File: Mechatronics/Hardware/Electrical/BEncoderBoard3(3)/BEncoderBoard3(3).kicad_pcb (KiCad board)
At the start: 4 copper layers, 34 x 33 mm, 10 parts, among them J1 Conn_01x04_Male, U8 RN4871U

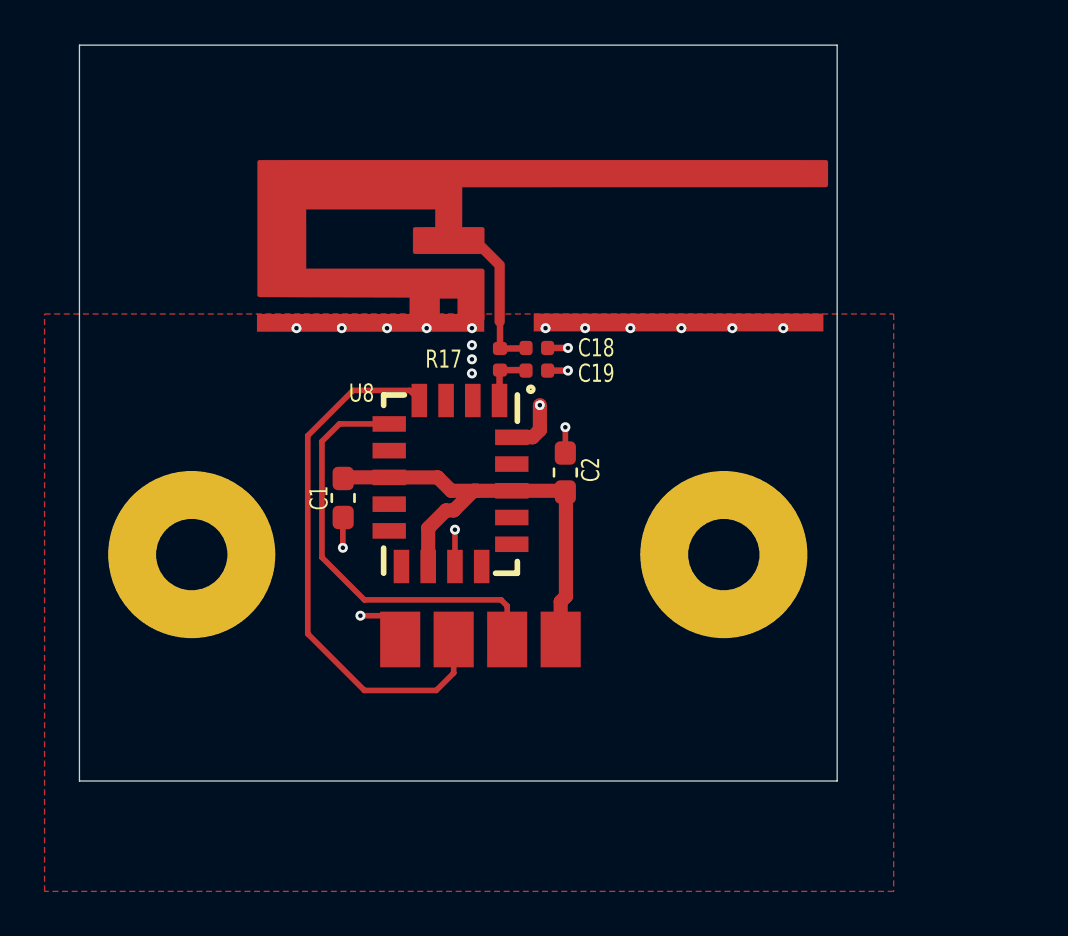
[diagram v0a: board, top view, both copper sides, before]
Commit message: PCB changes
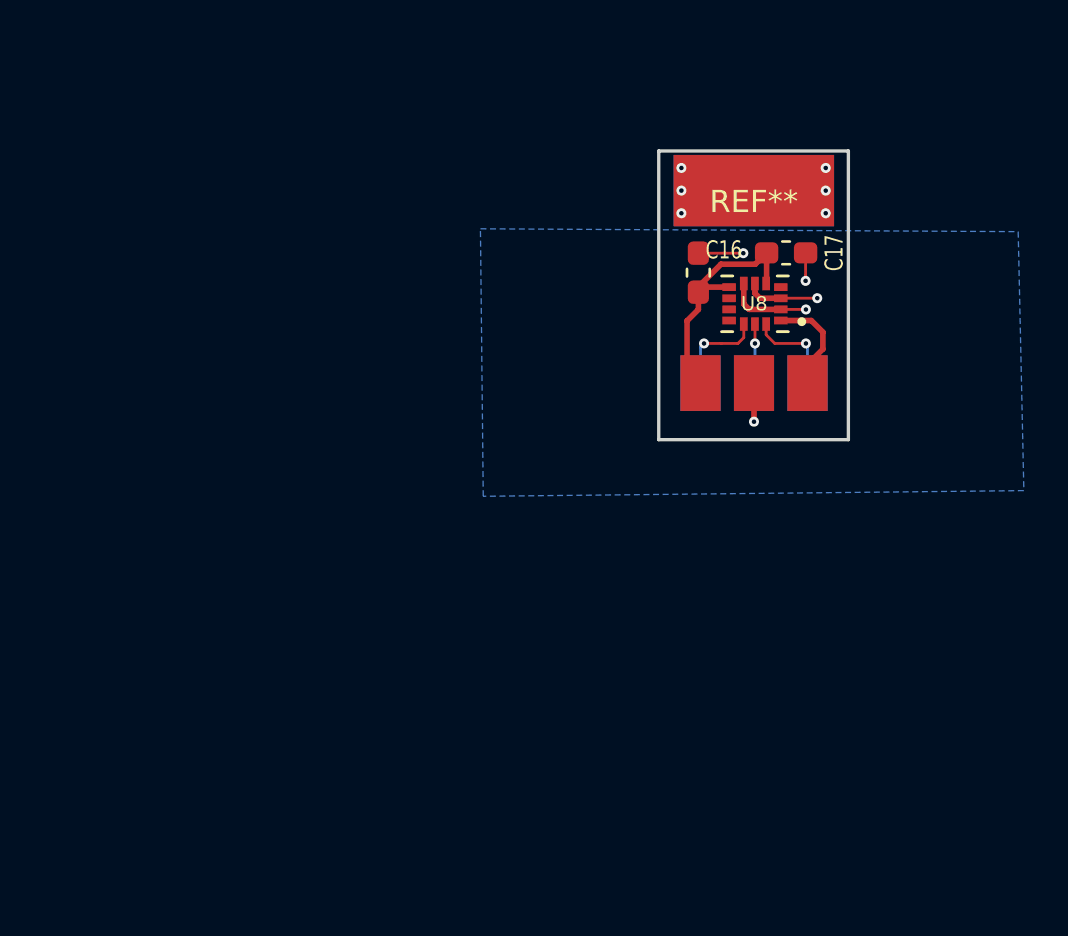
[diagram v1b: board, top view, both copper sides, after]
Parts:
- removed AE1: LOGO, Encoder:Antenna
- removed C1: 1uF, Encoder:C_0603_1608Metric_Pad1.05x0.95mm_HandSolder
- removed C18, C19: C_Rf, Encoder:C_0402_1005Metric
- removed C2: 10uF, Encoder:C_0603_1608Metric_Pad1.05x0.95mm_HandSolder
- removed R17: L_Rf, Encoder:L_0402_1005Metric
- removed the REF** at (121.5, 99.8)
- removed e: MountingHole_3.2mm_M3_Pad, Encoder:MountingHole_3.2mm_M3_Pad
- added C16: 100nF, Encoder:C_0603_1608Metric_Pad1.05x0.95mm_HandSolder, F.Cu at (144.3, 87.2)
- added C17: 100nF, Encoder:C_0603_1608Metric_Pad1.05x0.95mm_HandSolder, F.Cu at (148.2, 86.3)
- added REF**: TermicPad, Encoder:TermicPad, F.Cu at (146.8, 83.5)
- J1: value Conn_01x04_Male -> Conn_01x06_Male; footprint Encoder:SolderWirePad_1x04_SMD_5x10mm_copy -> Encoder:SolderWirePad_1x06_SMD_5x10mm
- U8: value RN4871U -> LSM6DSRX; footprint Encoder:RN4871U -> Encoder:LSM6DSRX
- moved U8 17.2 mm to (146.8, 88.6), turned to 180 degrees
- moved J1 16.9 mm to (146.8, 92.1)
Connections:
- J1 pad 1: GND -> /CS
- J1 pad 2: Net-(J1-Pad2) -> /SCL
- J1 pad 3: Net-(J1-Pad3) -> /SDA
- J1 pad 4: +3V3 -> /SDO
- U8 pad 1: Net-(C19-Pad1) -> /SDO
- U8 pad 11: +3V3 -> Net-(U9-Pad11)
- U8 pad 12: GND -> /CS
- U8 pad 13: Net-(U8-Pad13) -> /SCL
- U8 pad 14: Net-(U8-Pad14) -> /SDA
- U8 pad 2: Net-(U8-Pad2) -> GND
- U8 pad 3: Net-(U8-Pad3) -> GND
- U8 pad 4: Net-(J1-Pad2) -> Net-(U9-Pad4)
- U8 pad 5: Net-(J1-Pad3) -> +3V3
- U8 pad 6: Net-(U8-Pad6) -> GND
- U8 pad 7: +3V3 -> GND
- U8 pad 8: Net-(U8-Pad8) -> +3V3
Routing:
- net Net-(J1-Pad2): track 24.4 -> 0.00 mm
- net Net-(J1-Pad3): track 19.3 -> 0.00 mm
- net +3V3: track 21.7 -> 11.3 mm
- net /SDO: track 0.00 -> 4.68 mm
- net /CS: track 0.00 -> 4.34 mm, vias 0 -> 1
- net /SDA: track 0.00 -> 4.23 mm, vias 0 -> 1
- net /SCL: track 0.00 -> 2.66 mm, vias 0 -> 1
- net Net-(C19-Pad1): track 2.60 -> 0.00 mm
- net Net-(AE1-Pad1): track 2.33 -> 0.00 mm
- net GND: track 11.0 -> 12.1 mm, vias 21 -> 5
- net (no net): vias 0 -> 6
- added copper zone on B.Cu, net GND
- removed copper zone on F.Cu, net GND
- removed copper zone on In1.Cu, net GND
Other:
- board size 34 x 33 mm -> 8.5 x 13 mm
- copper layers 4 -> 2
- net class Default: clearance 0.1016 -> 0.127; trace_width 0.1016 -> 0.127
- rule trace_clearance: 0.1016 -> 0.127
- rule trace_min: 0.0889 -> 0.127
- rule via_min_size: 0.44 -> 0.45
